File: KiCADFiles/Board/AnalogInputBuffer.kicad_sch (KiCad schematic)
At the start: 18 parts, among them U15 OPA1655D, U16 OPA1655D

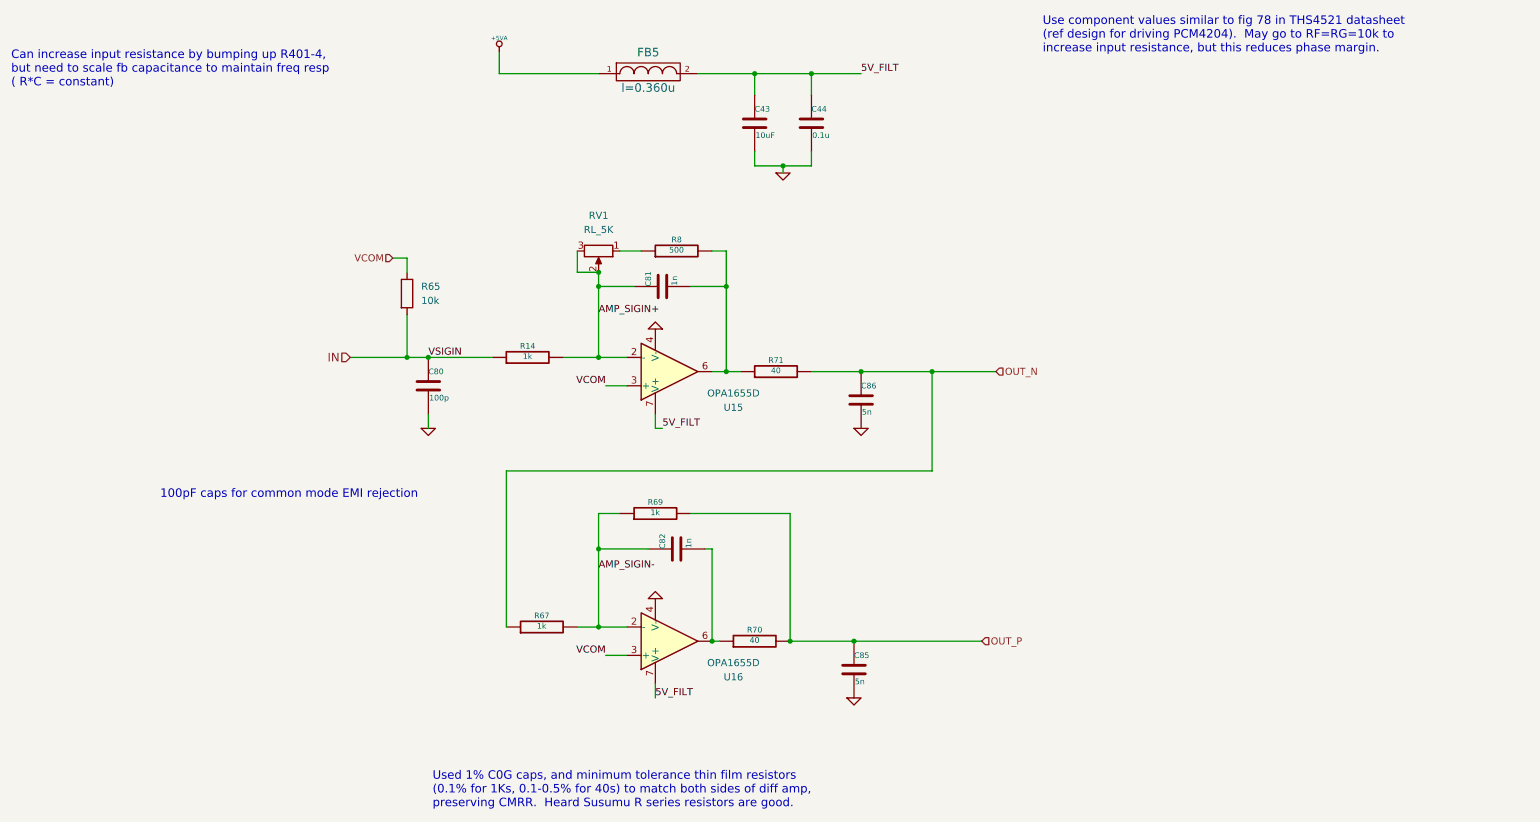
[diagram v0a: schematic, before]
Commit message: chose all components
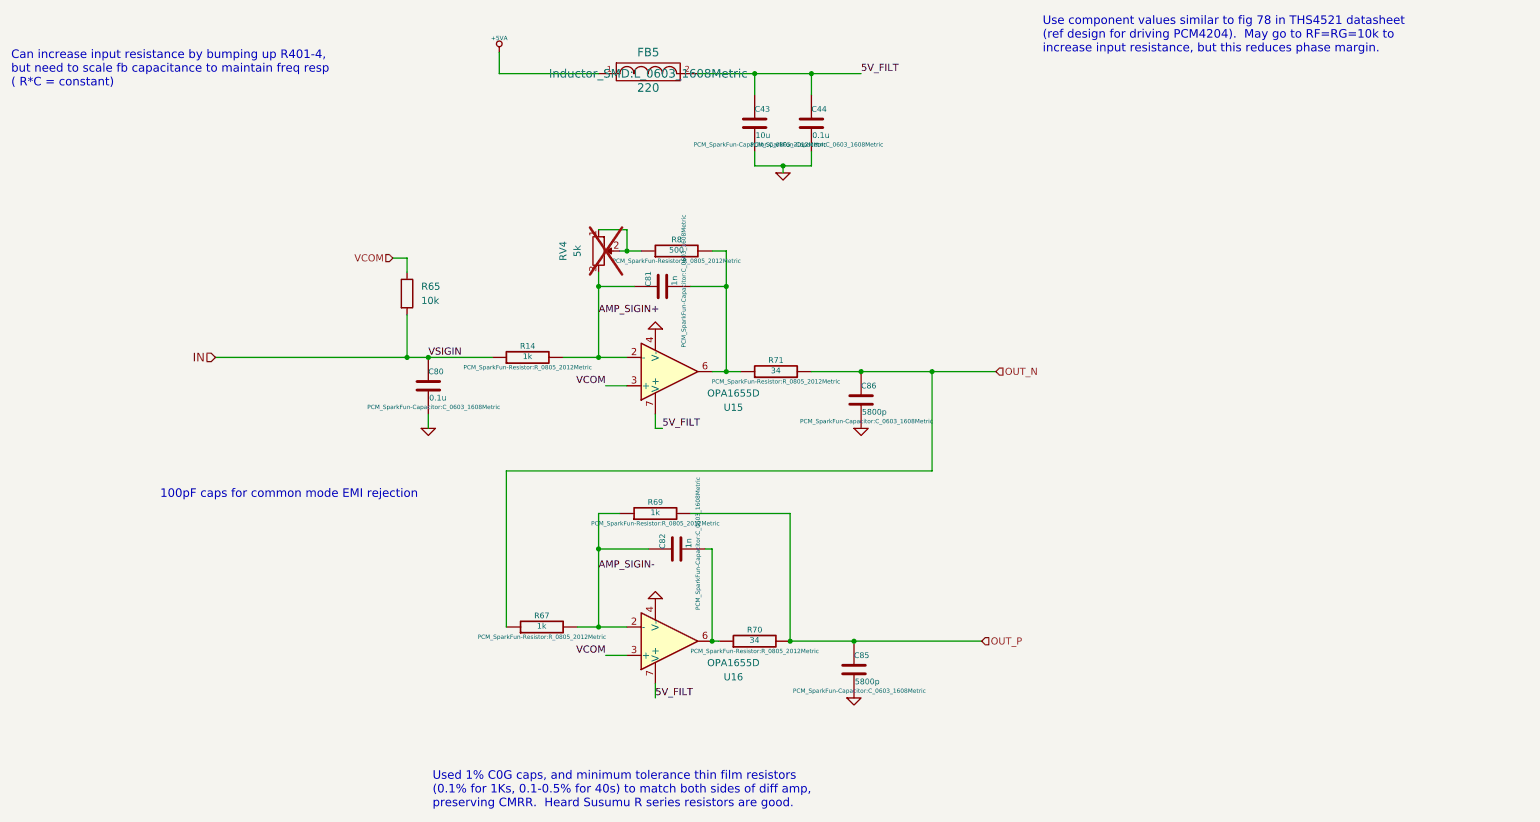
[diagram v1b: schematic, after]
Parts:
- removed RV1: RL_5K, symbol Device:R_Potentiometer
- added RV4: 5k, Potentiometer_THT:Potentiometer_Alps_RK163_Single_Horizontal, symbol Device:R_Potentiometer
- C43: value 10uF -> 10u; footprint ~ -> PCM_SparkFun-Capacitor:C_0805_2012Metric; MPN (none) -> CL21A106KAYNNNG; Voltage (none) -> 25V
- C44: footprint ~ -> PCM_SparkFun-Capacitor:C_0603_1608Metric; MPN (none) -> CL10B104KB8NNNL
- C80: value 100p -> 0.1u; footprint ~ -> PCM_SparkFun-Capacitor:C_0603_1608Metric; MPN (none) -> CL10B104KB8NNNL
- C81, C82: footprint ~ -> PCM_SparkFun-Capacitor:C_0603_1608Metric; MPN (none) -> GRM1885C1H102JA01D
- C85, C86: value 5n -> 5800p; footprint ~ -> PCM_SparkFun-Capacitor:C_0603_1608Metric; MPN (none) -> GCM1885C1H562GA16D
- FB5: value ${SIM.PARAMS} -> 220; footprint ~ -> Inductor_SMD:L_0603_1608Metric; MPN (none) -> MMZ1608B221CTAH0
- R14, R67, R69: footprint ~ -> PCM_SparkFun-Resistor:R_0805_2012Metric; MPN (none) -> ERA-6AEB102V
- R65: footprint (none) -> PCM_SparkFun-Resistor:R_0805_2012Metric; MPN (none) -> CRCW080510K0FKEA
- R70, R71: value 40 -> 34; footprint ~ -> PCM_SparkFun-Resistor:R_0805_2012Metric; MPN (none) -> CRCW080534R0FKEA
- R8: footprint ~ -> PCM_SparkFun-Resistor:R_0805_2012Metric; MPN (none) -> RMCF0805JT510R
- U15, U16: MPN (none) -> OPA1655D
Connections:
- net AMP_SIGIN+: now also RV4.3
- net at R8.1: now also RV4.1, RV4.2
